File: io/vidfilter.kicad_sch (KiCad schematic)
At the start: 14 parts

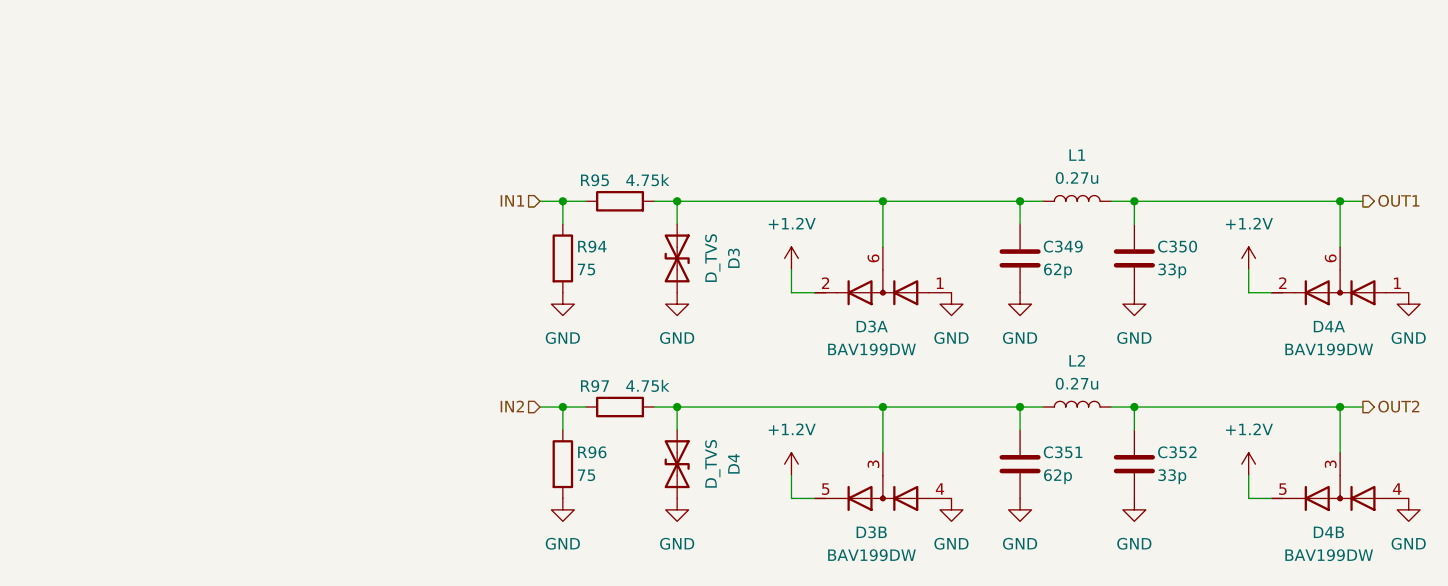
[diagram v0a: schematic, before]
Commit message: External I/O
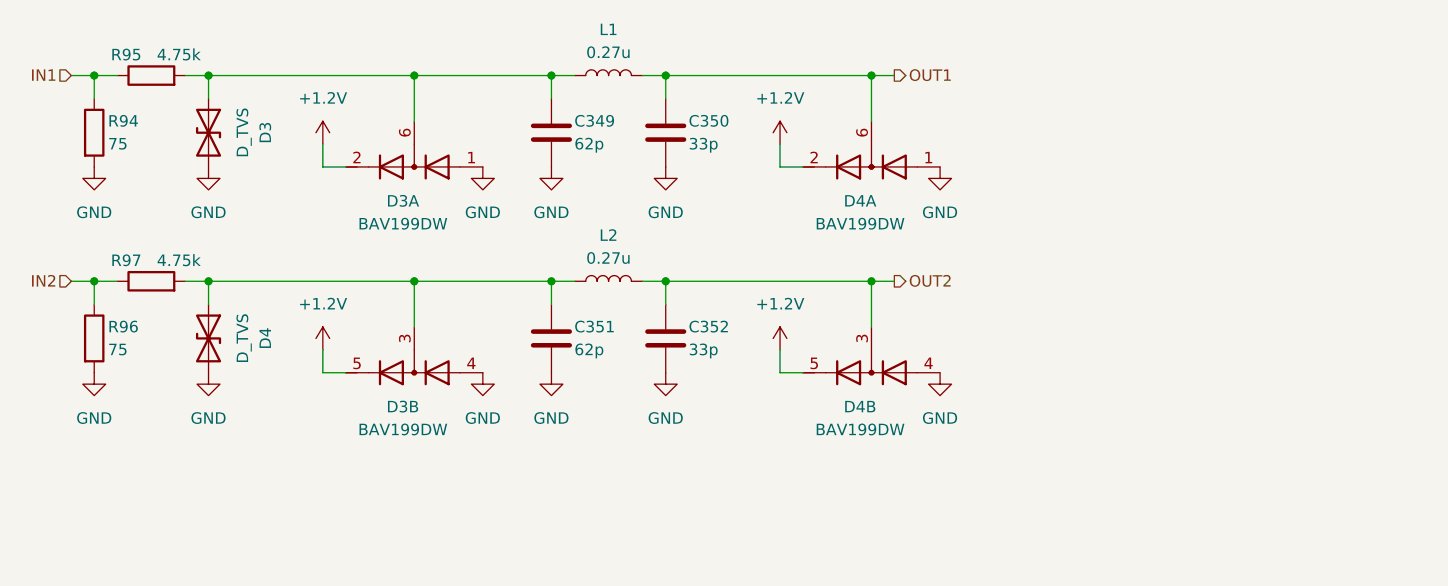
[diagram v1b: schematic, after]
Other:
- moved on the sheet: C349, C350, C351, C352, D3, D3A, D3B, D4, D4A, D4B, L1, L2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
